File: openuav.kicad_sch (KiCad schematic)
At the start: 71 parts, among them J1 Conn_01x01, J10 Conn_01x01, J11 Conn_01x01, J12 Conn_01x01, J13 Conn_01x01, J14 Conn_01x01, J15 Conn_01x01, J16 Conn_01x01, J17 Conn_01x01, J18 Conn_01x01, J19 Conn_01x01, J2 Conn_01x01, J20 Conn_01x01, J21 Conn_01x01, J22 Conn_01x01, J23 Conn_01x01, J24 Conn_01x01, J25 Conn_01x01, J26 Conn_01x01, J27 Conn_01x01, J28 Conn_01x01, J29 Conn_01x01, J3 Conn_01x01, J30 Conn_01x01, J31 Conn_01x01, J32 Conn_01x01, J33 Conn_01x01, J4 Conn_01x01, J5 Conn_01x01, J6 Conn_01x01, J7 Conn_01x01, J8 Conn_01x01, J9 Conn_01x01, J99 USB_C_Receptacle_USB2.0, SW1 SW_Push, U1 STM32G474CETx, U2 BMI270, U3 BMP280, U5 TPS54202DDC, U6 W25N01GVZEIG, U7 XC6206P332MR

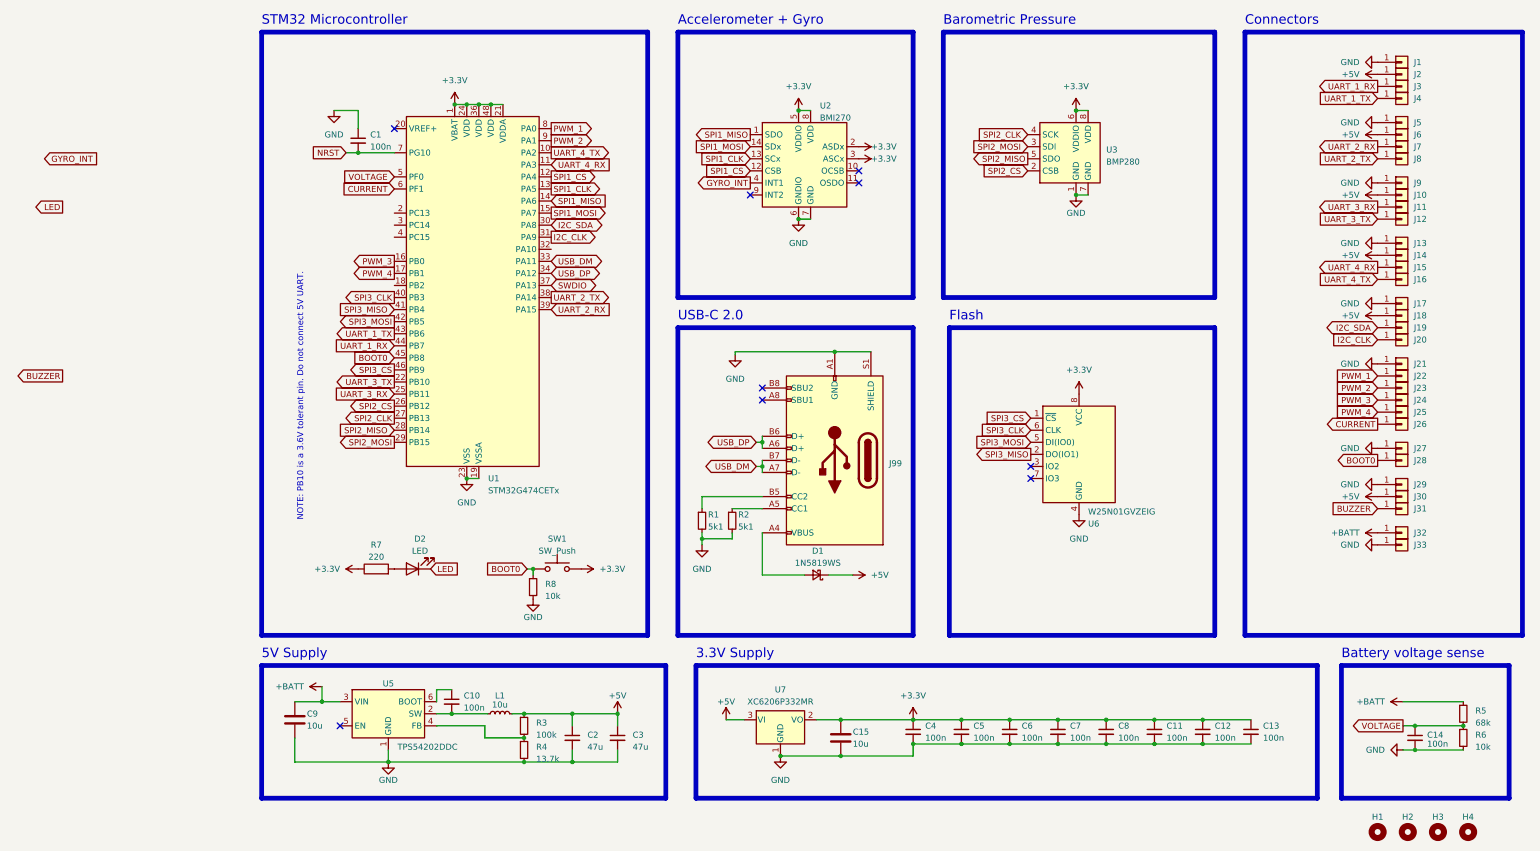
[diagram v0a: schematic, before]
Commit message: continue g474 redesign
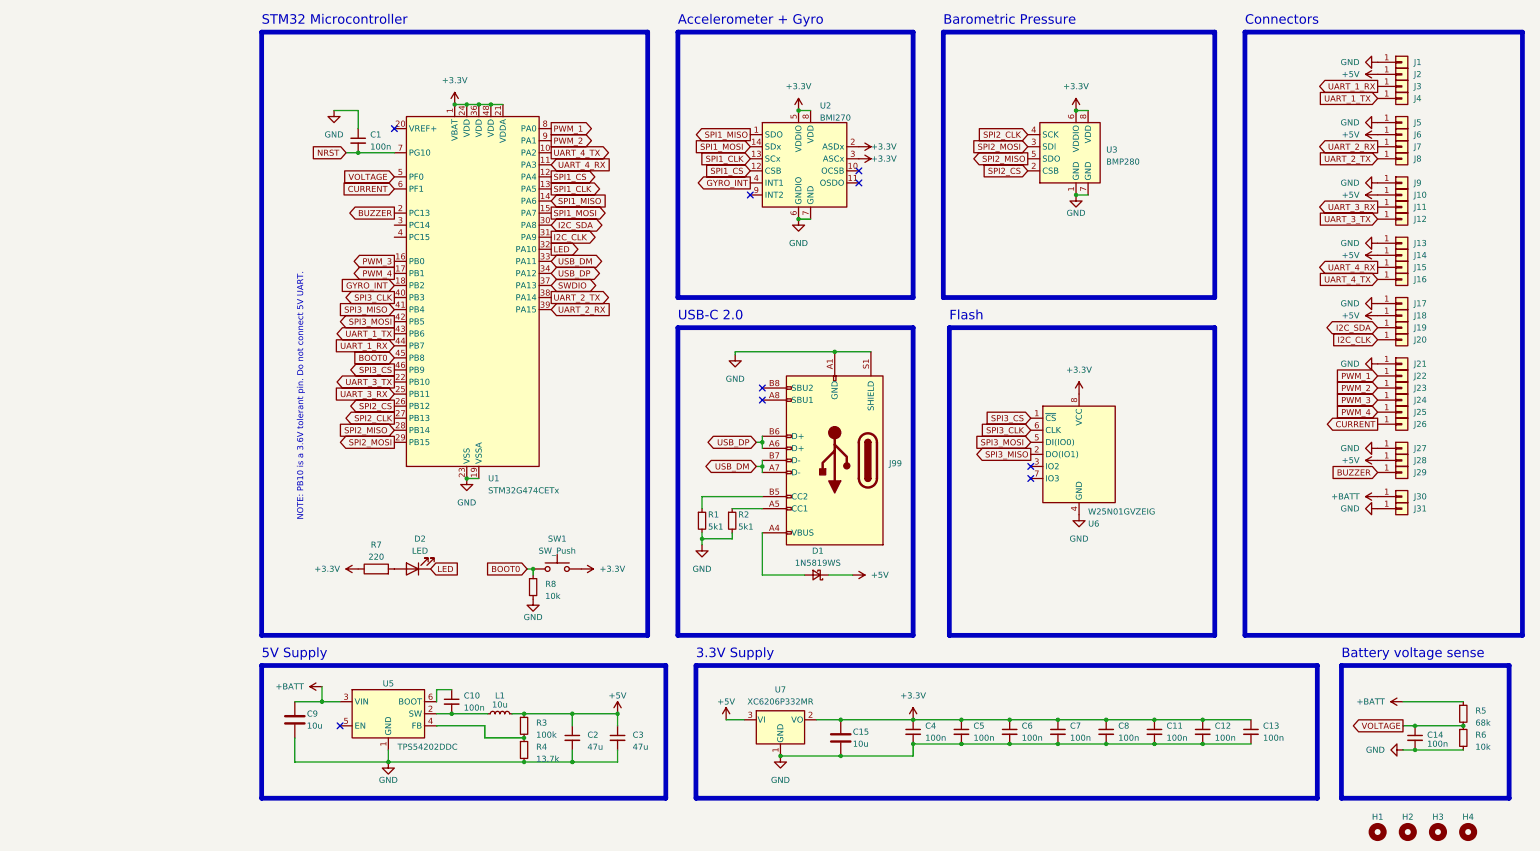
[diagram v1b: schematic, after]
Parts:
- removed J32, J33: Conn_01x01, Connector_Custom_Pads:TP-2.54, symbol Connector_Generic:Conn_01x01
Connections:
- net +5V: now also J28.1 (Pin_1); no longer J30.1 (Pin_1)
- net +BATT: now also J30.1 (Pin_1)
- net BOOT0: no longer J28.1 (Pin_1)
- net BUZZER: now also J29.1 (Pin_1), U1.2 (PC13); no longer J31.1 (Pin_1)
- net GND: now also J31.1 (Pin_1); no longer J29.1 (Pin_1)
- net GYRO_INT: now also U1.18 (PB2)
- net LED: now also U1.32 (PA10)
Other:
- moved on the sheet: J29

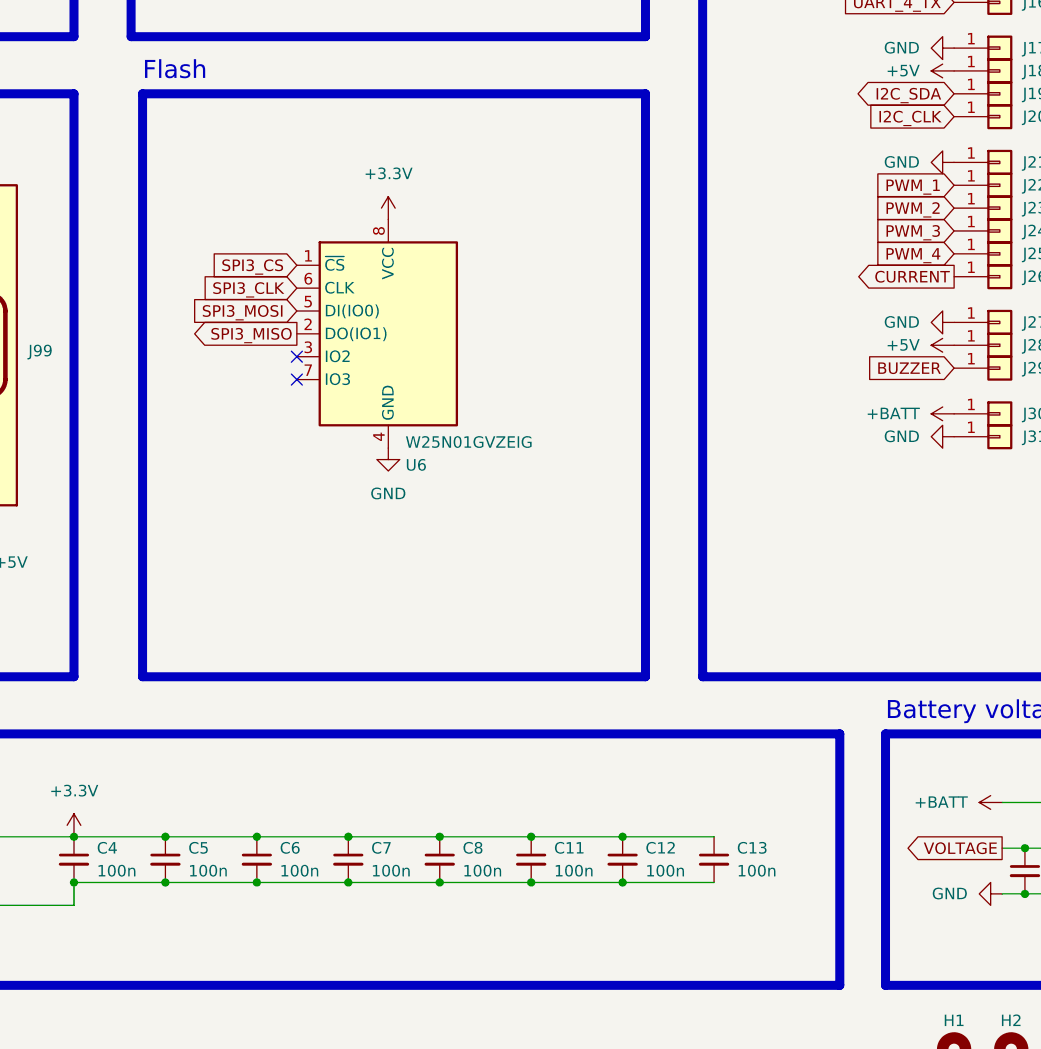
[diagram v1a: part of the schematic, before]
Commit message: continued work on G474 board
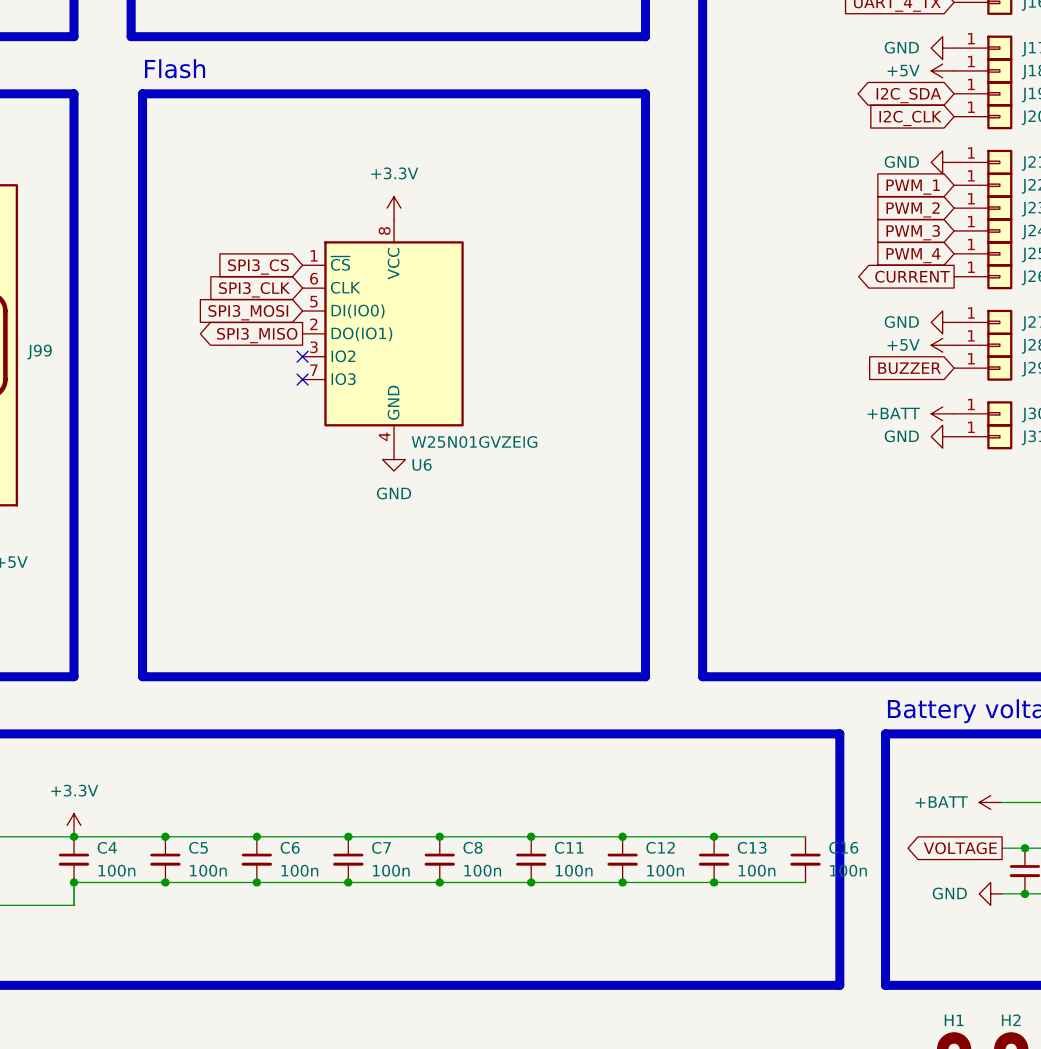
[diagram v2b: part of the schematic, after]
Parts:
- added C16: 100n, Capacitor_SMD:C_0402_1005Metric, symbol Device:C_Small
- L1: footprint Inductor_SMD:L_Sunlord_MWSA0603S -> Inductor_SMD:L_Sunlord_MWSA0402S; LCSC C132141 -> C408339
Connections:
- net +3V3: now also C16.1
- net GND: now also C16.2
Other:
- moved on the sheet: U6
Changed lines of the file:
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@@
   (junction (at 59.69 39.37) (diameter 0) (color 0 0 0 0)
   )
+  (junction (at 224.79 168.91) (diameter 0) (color 0 0 0 0)
+  )
   (junction (at 121.92 115.57) (diameter 0) (color 0 0 0 0)
   )
@@
   (junction (at 214.63 173.99) (diameter 0) (color 0 0 0 0)
   )
+  (junction (at 224.79 173.99) (diameter 0) (color 0 0 0 0)
+  )
   (junction (at 71.755 172.72) (diameter 0) (color 0 0 0 0)
   )
@@
   (no_connect (at 44.45 44.45))
   (no_connect (at 142.24 55.88))
-  (no_connect (at 178.435 118.11))
+  (no_connect (at 179.07 118.11))
   (no_connect (at 121.92 99.06))
   (no_connect (at 142.24 53.34))
   (no_connect (at 121.92 101.6))
   (no_connect (at 119.38 58.42))
-  (no_connect (at 178.435 115.57))
+  (no_connect (at 179.07 115.57))
   (no_connect (at 33.02 170.18))
   (wire (pts (xy 36.83 49.53) (xy 44.45 49.53))
@@
     (stroke (width 0) (type default))
   )
+  (wire (pts (xy 224.79 173.99) (xy 234.95 173.99))
+    (stroke (width 0) (type default))
+  )
   (wire (pts (xy 63.5 170.18) (xy 63.5 172.72))
     (stroke (width 0) (type default))
@@
     (stroke (width 0) (type default))
   )
+  (wire (pts (xy 224.79 168.91) (xy 234.95 168.91))
+    (stroke (width 0) (type default))
+  )
   (wire (pts (xy 81.915 177.8) (xy 91.44 177.8))
     (stroke (width 0) (type default))
@@
     )
   )
-  (global_label "SPI3_CS" (shape input) (at 178.435 105.41 180) (fields_autoplaced)
+  (global_label "SPI3_CS" (shape input) (at 179.07 105.41 180) (fields_autoplaced)
     (effects (font (size 1.27 1.27)) (justify right))
-    (property "Intersheetrefs" "${INTERSHEET_REFS}" (at 167.7883 105.41 0)
+    (property "Intersheetrefs" "${INTERSHEET_REFS}" (at 168.4233 105.41 0)
       (effects (font (size 1.27 1.27)) (justify right) hide)
     )
@@
     )
   )
-  (global_label "SPI3_MOSI" (shape input) (at 178.435 110.49 180) (fields_autoplaced)
+  (global_label "SPI3_MOSI" (shape input) (at 179.07 110.49 180) (fields_autoplaced)
     (effects (font (size 1.27 1.27)) (justify right))
-    (property "Intersheetrefs" "${INTERSHEET_REFS}" (at 165.6716 110.49 0)
+    (property "Intersheetrefs" "${INTERSHEET_REFS}" (at 166.3066 110.49 0)
       (effects (font (size 1.27 1.27)) (justify right) hide)
     )
@@
     )
   )
-  (global_label "SPI3_MISO" (shape output) (at 178.435 113.03 180) (fields_autoplaced)
+  (global_label "SPI3_MISO" (shape output) (at 179.07 113.03 180) (fields_autoplaced)
     (effects (font (size 1.27 1.27)) (justify right))
-    (property "Intersheetrefs" "${INTERSHEET_REFS}" (at 165.6716 113.03 0)
+    (property "Intersheetrefs" "${INTERSHEET_REFS}" (at 166.3066 113.03 0)
       (effects (font (size 1.27 1.27)) (justify right) hide)
     )
@@
     )
   )
-  (global_label "SPI3_CLK" (shape input) (at 178.435 107.95 180) (fields_autoplaced)
+  (global_label "SPI3_CLK" (shape input) (at 179.07 107.95 180) (fields_autoplaced)
     (effects (font (size 1.27 1.27)) (justify right))
-    (property "Intersheetrefs" "${INTERSHEET_REFS}" (at 166.6997 107.95 0)
+    (property "Intersheetrefs" "${INTERSHEET_REFS}" (at 167.3347 107.95 0)
       (effects (font (size 1.27 1.27)) (justify right) hide)
     )
@@
     )
   )
-  (symbol (lib_id "Memory_Flash:W25Q32JVSS") (at 188.595 113.03 0) (unit 1)
+  (symbol (lib_id "Memory_Flash:W25Q32JVSS") (at 189.23 113.03 0) (unit 1)
     (in_bom yes) (on_board yes) (dnp no)
-    (property "Reference" "U6" (at 190.5 127.635 0)
+    (property "Reference" "U6" (at 191.135 127.635 0)
       (effects (font (size 1.27 1.27)) (justify left))
     )
-    (property "Value" "W25N01GVZEIG" (at 190.5 125.095 0)
+    (property "Value" "W25N01GVZEIG" (at 191.135 125.095 0)
       (effects (font (size 1.27 1.27)) (justify left))
     )
-    (property "Footprint" "Package_SON:WSON-8-1EP_8x6mm_P1.27mm_EP3.4x4.3mm" (at 188.595 113.03 0)
+    (property "Footprint" "Package_SON:WSON-8-1EP_8x6mm_P1.27mm_EP3.4x4.3mm" (at 189.23 113.03 0)
       (effects (font (size 1.27 1.27)) hide)
     )
-    (property "Datasheet" "http://www.winbond.com/resource-files/w25q32jv%20revg%2003272018%20plus.pdf" (at 188.595 113.03 0)
+    (property "Datasheet" "http://www.winbond.com/resource-files/w25q32jv%20revg%2003272018%20plus.pdf" (at 189.23 113.03 0)
       (effects (font (size 1.27 1.27)) hide)
     )
-    (property "LCSC" "C88868" (at 188.595 113.03 0)
+    (property "LCSC" "C88868" (at 189.23 113.03 0)
       (effects (font (size 1.27 1.27)) hide)
     )
@@
       (effects (font (size 1.27 1.27)))
     )
-    (property "Footprint" "Inductor_SMD:L_Sunlord_MWSA0603S" (at 66.675 167.64 0)
+    (property "Footprint" "Inductor_SMD:L_Sunlord_MWSA0402S" (at 66.675 167.64 0)
       (effects (font (size 1.27 1.27)) hide)
     )
@@
       (effects (font (size 1.27 1.27)) hide)
     )
-    (property "LCSC" "C132141" (at 66.675 167.64 0)
+    (property "LCSC" "C408339" (at 66.675 167.64 0)
       (effects (font (size 1.27 1.27)) hide)
     )
@@
     )
   )
-  (symbol (lib_id "power:+3.3V") (at 188.595 100.33 0) (unit 1)
+  (symbol (lib_id "power:+3.3V") (at 189.23 100.33 0) (unit 1)
     (in_bom yes) (on_board yes) (dnp no) (fields_autoplaced)
-    (property "Reference" "#PWR01" (at 188.595 104.14 0)
+    (property "Reference" "#PWR01" (at 189.23 104.14 0)
       (effects (font (size 1.27 1.27)) hide)
     )
-    (property "Value" "+3.3V" (at 188.595 95.25 0)
+    (property "Value" "+3.3V" (at 189.23 95.25 0)
       (effects (font (size 1.27 1.27)))
     )
-    (property "Footprint" "" (at 188.595 100.33 0)
+    (property "Footprint" "" (at 189.23 100.33 0)
       (effects (font (size 1.27 1.27)) hide)
     )
-    (property "Datasheet" "" (at 188.595 100.33 0)
+    (property "Datasheet" "" (at 189.23 100.33 0)
       (effects (font (size 1.27 1.27)) hide)
     )
@@
     )
   )
-  (symbol (lib_id "power:GND") (at 188.595 125.73 0) (unit 1)
+  (symbol (lib_id "power:GND") (at 189.23 125.73 0) (unit 1)
     (in_bom yes) (on_board yes) (dnp no) (fields_autoplaced)
-    (property "Reference" "#PWR03" (at 188.595 132.08 0)
+    (property "Reference" "#PWR03" (at 189.23 132.08 0)
       (effects (font (size 1.27 1.27)) hide)
     )
-    (property "Value" "GND" (at 188.595 130.81 0)
+    (property "Value" "GND" (at 189.23 130.81 0)
       (effects (font (size 1.27 1.27)))
     )
-    (property "Footprint" "" (at 188.595 125.73 0)
+    (property "Footprint" "" (at 189.23 125.73 0)
       (effects (font (size 1.27 1.27)) hide)
     )
-    (property "Datasheet" "" (at 188.595 125.73 0)
+    (property "Datasheet" "" (at 189.23 125.73 0)
       (effects (font (size 1.27 1.27)) hide)
     )
@@
         )
       )
+    )
+  )
+  (symbol (lib_id "Device:C_Small") (at 234.95 171.45 0) (unit 1)
+    (in_bom yes) (on_board yes) (dnp no) (fields_autoplaced)
+    (property "Reference" "C16" (at 237.49 170.1862 0)
+      (effects (font (size 1.27 1.27)) (justify left))
+    )
+    (property "Value" "100n" (at 237.49 172.7262 0)
+      (effects (font (size 1.27 1.27)) (justify left))
+    )
+    (property "Footprint" "Capacitor_SMD:C_0402_1005Metric" (at 234.95 171.45 0)
+      (effects (font (size 1.27 1.27)) hide)
+    )
+    (property "Datasheet" "~" (at 234.95 171.45 0)
+      (effects (font (size 1.27 1.27)) hide)
+    )
+    (property "LCSC" "C307331" (at 234.95 171.45 0)
+      (effects (font (size 1.27 1.27)) hide)
+    )
+    (pin "1")
+    (pin "2")
+    (instances
+      (project "openuav"
+        (path "/e63e39d7-6ac0-4ffd-8aa3-1841a4541b55"
+          (reference "C16") (unit 1)
+        )
+      )
